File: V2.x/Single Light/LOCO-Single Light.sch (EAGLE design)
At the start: 32 parts, among them IC1 Atmega 328-P, IC2 MCP2515, IC3 MIC5219BM5, Q1 8MHz, Q2 16MHz

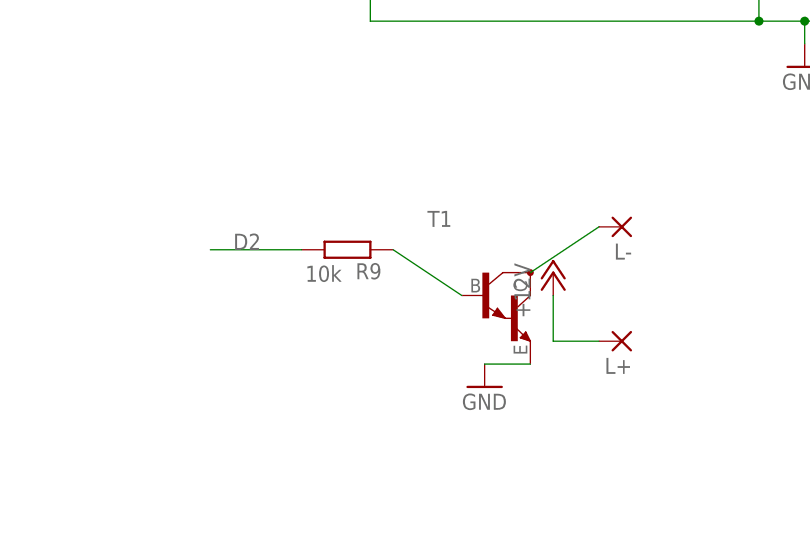
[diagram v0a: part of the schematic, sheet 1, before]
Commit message: initial
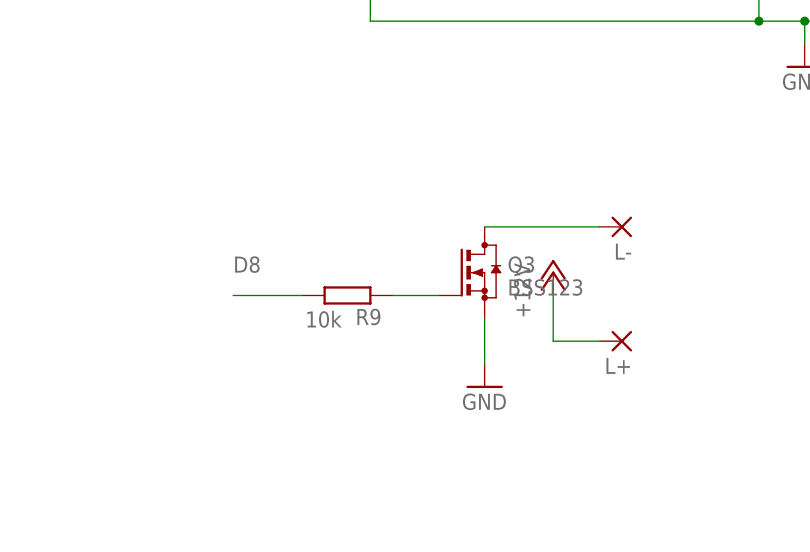
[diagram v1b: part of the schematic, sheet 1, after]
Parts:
- removed T1: (no value), transistor-neu-to92:MMBTA13LT1-NPN_DARL-SOT23-BEC
- added Q3: BSS123, transistor-small-signal:BSS123
- Q1, Q2: device crystal:CRYSTALHC49S -> crystal-geyer_V1_0:KX-9B
- R1, R15, R2, R9: device rcl:R-EU_R0603 -> rcl:R-EU_R0402
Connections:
- net D2: no longer R9.2
- net D8: now also R9.2
- net GND: now also Q3.S; no longer T1.E
- net LIGHT: now also Q3.D; no longer T1.C
- net N$2: now also Q3.G; no longer T1.B
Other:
- moved on the sheet: R9
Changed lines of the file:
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@@
 <part name="GND2" library="supply1" library_urn="urn:adsk.eagle:library:371" deviceset="GND" device=""/>
 <part name="P+2" library="supply1" library_urn="urn:adsk.eagle:library:371" deviceset="VCC" device=""/>
-<part name="R1" library="rcl" library_urn="urn:adsk.eagle:library:334" deviceset="R-EU_" device="R0603" package3d_urn="urn:adsk.eagle:package:23555/3" value="10k"/>
+<part name="R1" library="rcl" library_urn="urn:adsk.eagle:library:334" deviceset="R-EU_" device="R0402" package3d_urn="urn:adsk.eagle:package:23547/3" value="10k"/>
 <part name="C1" library="rcl" library_urn="urn:adsk.eagle:library:334" deviceset="C-EU" device="C0402K" package3d_urn="urn:adsk.eagle:package:23679/2" value="22p"/>
 <part name="C2" library="rcl" library_urn="urn:adsk.eagle:library:334" deviceset="C-EU" device="C0402K" package3d_urn="urn:adsk.eagle:package:23679/2" value="22p"/>
 <part name="GND3" library="supply1" library_urn="urn:adsk.eagle:library:371" deviceset="GND" device=""/>
-<part name="Q1" library="crystal" library_urn="urn:adsk.eagle:library:204" deviceset="CRYSTAL" device="HC49S" package3d_urn="urn:adsk.eagle:package:12071/1" value="8MHz"/>
+<part name="Q1" library="crystal-geyer_V1_0" library_urn="urn:adsk.eagle:library:203" deviceset="KX" device="-9B" package3d_urn="urn:adsk.eagle:package:11930/1" value="8MHz"/>
 <part name="C3" library="rcl" library_urn="urn:adsk.eagle:library:334" deviceset="C-EU" device="C0402K" package3d_urn="urn:adsk.eagle:package:23679/2" value="22p"/>
 <part name="C4" library="rcl" library_urn="urn:adsk.eagle:library:334" deviceset="C-EU" device="C0402K" package3d_urn="urn:adsk.eagle:package:23679/2" value="22p"/>
 <part name="GND4" library="supply1" library_urn="urn:adsk.eagle:library:371" deviceset="GND" device=""/>
-<part name="Q2" library="crystal" library_urn="urn:adsk.eagle:library:204" deviceset="CRYSTAL" device="HC49S" package3d_urn="urn:adsk.eagle:package:12071/1" value="16MHz"/>
-<part name="R2" library="rcl" library_urn="urn:adsk.eagle:library:334" deviceset="R-EU_" device="R0603" package3d_urn="urn:adsk.eagle:package:23555/3" value="10k"/>
+<part name="Q2" library="crystal-geyer_V1_0" library_urn="urn:adsk.eagle:library:203" deviceset="KX" device="-9B" package3d_urn="urn:adsk.eagle:package:11930/1" value="16MHz"/>
+<part name="R2" library="rcl" library_urn="urn:adsk.eagle:library:334" deviceset="R-EU_" device="R0402" package3d_urn="urn:adsk.eagle:package:23547/3" value="10k"/>
 <part name="C5" library="rcl" library_urn="urn:adsk.eagle:library:334" deviceset="C-EU" device="C0402K" package3d_urn="urn:adsk.eagle:package:23679/2" value="100n"/>
 <part name="IC1" library="atmel" library_urn="urn:adsk.eagle:library:105" deviceset="MEGA8" device="-AI" package3d_urn="urn:adsk.eagle:package:4313/2" value="Atmega 328-P"/>
@@
 <part name="C16" library="rcl" library_urn="urn:adsk.eagle:library:334" deviceset="CPOL-EU" device="A/3216-18W" package3d_urn="urn:adsk.eagle:package:23408/2" value="16uF"/>
 <part name="GND8" library="supply1" library_urn="urn:adsk.eagle:library:371" deviceset="GND" device=""/>
-<part name="R9" library="rcl" library_urn="urn:adsk.eagle:library:334" deviceset="R-EU_" device="R0603" package3d_urn="urn:adsk.eagle:package:23555/3" value="10k"/>
-<part name="R15" library="rcl" library_urn="urn:adsk.eagle:library:334" deviceset="R-EU_" device="R0603" package3d_urn="urn:adsk.eagle:package:23555/3" value="10k"/>
+<part name="R9" library="rcl" library_urn="urn:adsk.eagle:library:334" deviceset="R-EU_" device="R0402" package3d_urn="urn:adsk.eagle:package:23547/3" value="10k"/>
+<part name="R15" library="rcl" library_urn="urn:adsk.eagle:library:334" deviceset="R-EU_" device="R0402" package3d_urn="urn:adsk.eagle:package:23547/3" value="10k"/>
 <part name="+5V" library="led" library_urn="urn:adsk.eagle:library:259" deviceset="LED" device="CHIP-LED0603" package3d_urn="urn:adsk.eagle:package:15819/3"/>
 <part name="P+4" library="supply1" library_urn="urn:adsk.eagle:library:371" deviceset="+12V" device=""/>
@@
 <part name="L-" library="wirepad" library_urn="urn:adsk.eagle:library:412" deviceset="1,6/0,8" device="" package3d_urn="urn:adsk.eagle:package:30830/1"/>
 <part name="L+" library="wirepad" library_urn="urn:adsk.eagle:library:412" deviceset="1,6/0,8" device="" package3d_urn="urn:adsk.eagle:package:30830/1"/>
-<part name="T1" library="transistor-neu-to92" library_urn="urn:adsk.eagle:library:397" deviceset="*-NPN_DARL-" device="SOT23-BEC" package3d_urn="urn:adsk.eagle:package:28748/2" technology="MMBTA13LT1"/>
 <part name="GND5" library="supply1" library_urn="urn:adsk.eagle:library:371" deviceset="GND" device=""/>
 <part name="C-G" library="wirepad" library_urn="urn:adsk.eagle:library:412" deviceset="1,6/0,8" device="" package3d_urn="urn:adsk.eagle:package:30830/1"/>
@@
 <part name="IC3" library="v-reg-micrel" library_urn="urn:adsk.eagle:library:408" deviceset="MIC5219BM5" device="" package3d_urn="urn:adsk.eagle:package:30272/1"/>
 <part name="C7" library="rcl" library_urn="urn:adsk.eagle:library:334" deviceset="C-EU" device="C0402K" package3d_urn="urn:adsk.eagle:package:23679/2" value="470pF"/>
+<part name="Q3" library="transistor-small-signal" library_urn="urn:adsk.eagle:library:401" deviceset="BSS123" device="" package3d_urn="urn:adsk.eagle:package:28738/2"/>
 </parts>
 <sheets>
@@
 <attribute name="VALUE" x="53.34" y="-60.96" size="1.778" layer="96"/>
 </instance>
-<instance part="R9" gate="G$1" x="101.6" y="-30.48" smashed="yes" rot="R180" grouprefs="FET">
-<attribute name="NAME" x="105.41" y="-31.9786" size="1.778" layer="95" rot="R180"/>
-<attribute name="VALUE" x="100.965" y="-32.258" size="1.778" layer="96" rot="R180"/>
+<instance part="R9" gate="G$1" x="101.6" y="-35.56" smashed="yes" rot="R180" grouprefs="FET">
+<attribute name="NAME" x="105.41" y="-37.0586" size="1.778" layer="95" rot="R180"/>
+<attribute name="VALUE" x="100.965" y="-37.338" size="1.778" layer="96" rot="R180"/>
 </instance>
 <instance part="R15" gate="G$1" x="55.88" y="-45.72" smashed="yes" rot="R90" grouprefs="POWER">
@@
 <attribute name="VALUE" x="133.223" y="-37.338" size="1.778" layer="96" rot="R180"/>
 </instance>
-<instance part="T1" gate="G$1" x="116.84" y="-35.56" smashed="yes">
-<attribute name="NAME" x="110.49" y="-27.94" size="1.778" layer="95"/>
-<attribute name="VALUE" x="112.776" y="-30.48" size="1.778" layer="96"/>
-</instance>
 <instance part="GND5" gate="1" x="116.84" y="-45.72" smashed="yes" grouprefs="FET">
 <attribute name="VALUE" x="114.3" y="-48.26" size="1.778" layer="96"/>
@@
 <attribute name="NAME" x="-4.064" y="-46.101" size="1.778" layer="95" rot="R180"/>
 <attribute name="VALUE" x="-4.064" y="-41.021" size="1.778" layer="96" rot="R180"/>
+</instance>
+<instance part="Q3" gate="G$1" x="116.84" y="-33.02" smashed="yes">
+<attribute name="NAME" x="119.38" y="-33.02" size="1.778" layer="95"/>
+<attribute name="VALUE" x="119.38" y="-35.56" size="1.778" layer="96"/>
 </instance>
 </instances>
@@
 </segment>
 <segment>
-<wire x1="121.92" y1="-43.18" x2="116.84" y2="-43.18" width="0.1524" layer="91" grouprefs="FET"/>
-<pinref part="T1" gate="G$1" pin="E"/>
+<wire x1="116.84" y1="-38.1" x2="116.84" y2="-43.18" width="0.1524" layer="91" grouprefs="FET"/>
 <pinref part="GND5" gate="1" pin="GND"/>
+<pinref part="Q3" gate="G$1" pin="S"/>
 </segment>
 </net>
@@
 <pinref part="IC1" gate="G$1" pin="PB0(ICP)"/>
 </segment>
+<segment>
+<pinref part="R9" gate="G$1" pin="2"/>
+<wire x1="96.52" y1="-35.56" x2="88.9" y2="-35.56" width="0.1524" layer="91" grouprefs="FET"/>
+<label x="88.9" y="-33.02" size="1.778" layer="95" grouprefs="FET"/>
+</segment>
 </net>
 <net name="TX" class="0">
@@
 <wire x1="58.42" y1="45.72" x2="73.66" y2="45.72" width="0.1524" layer="91" grouprefs="MCU"/>
 <label x="68.58" y="45.72" size="1.778" layer="95" grouprefs="MCU"/>
-</segment>
-<segment>
-<pinref part="R9" gate="G$1" pin="2"/>
-<wire x1="96.52" y1="-30.48" x2="86.36" y2="-30.48" width="0.1524" layer="91" grouprefs="FET"/>
-<label x="88.9" y="-30.48" size="1.778" layer="95" grouprefs="FET"/>
 </segment>
 </net>
@@
 <net name="N$2" class="0">
 <segment>
-<wire x1="114.3" y1="-35.56" x2="106.68" y2="-30.48" width="0.1524" layer="91" grouprefs="FET"/>
+<wire x1="111.76" y1="-35.56" x2="106.68" y2="-35.56" width="0.1524" layer="91" grouprefs="FET"/>
 <pinref part="R9" gate="G$1" pin="1"/>
-<pinref part="T1" gate="G$1" pin="B"/>
+<pinref part="Q3" gate="G$1" pin="G"/>
 </segment>
 </net>
@@
 <net name="LIGHT" class="0">
 <segment>
-<wire x1="121.92" y1="-33.02" x2="129.54" y2="-27.94" width="0.1524" layer="91" grouprefs="FET"/>
+<wire x1="116.84" y1="-27.94" x2="129.54" y2="-27.94" width="0.1524" layer="91" grouprefs="FET"/>
 <pinref part="L-" gate="P" pin="P"/>
-<pinref part="T1" gate="G$1" pin="C"/>
-</segment>
-</net>
+<pinref part="Q3" gate="G$1" pin="D"/>
+</segment>
+</net>

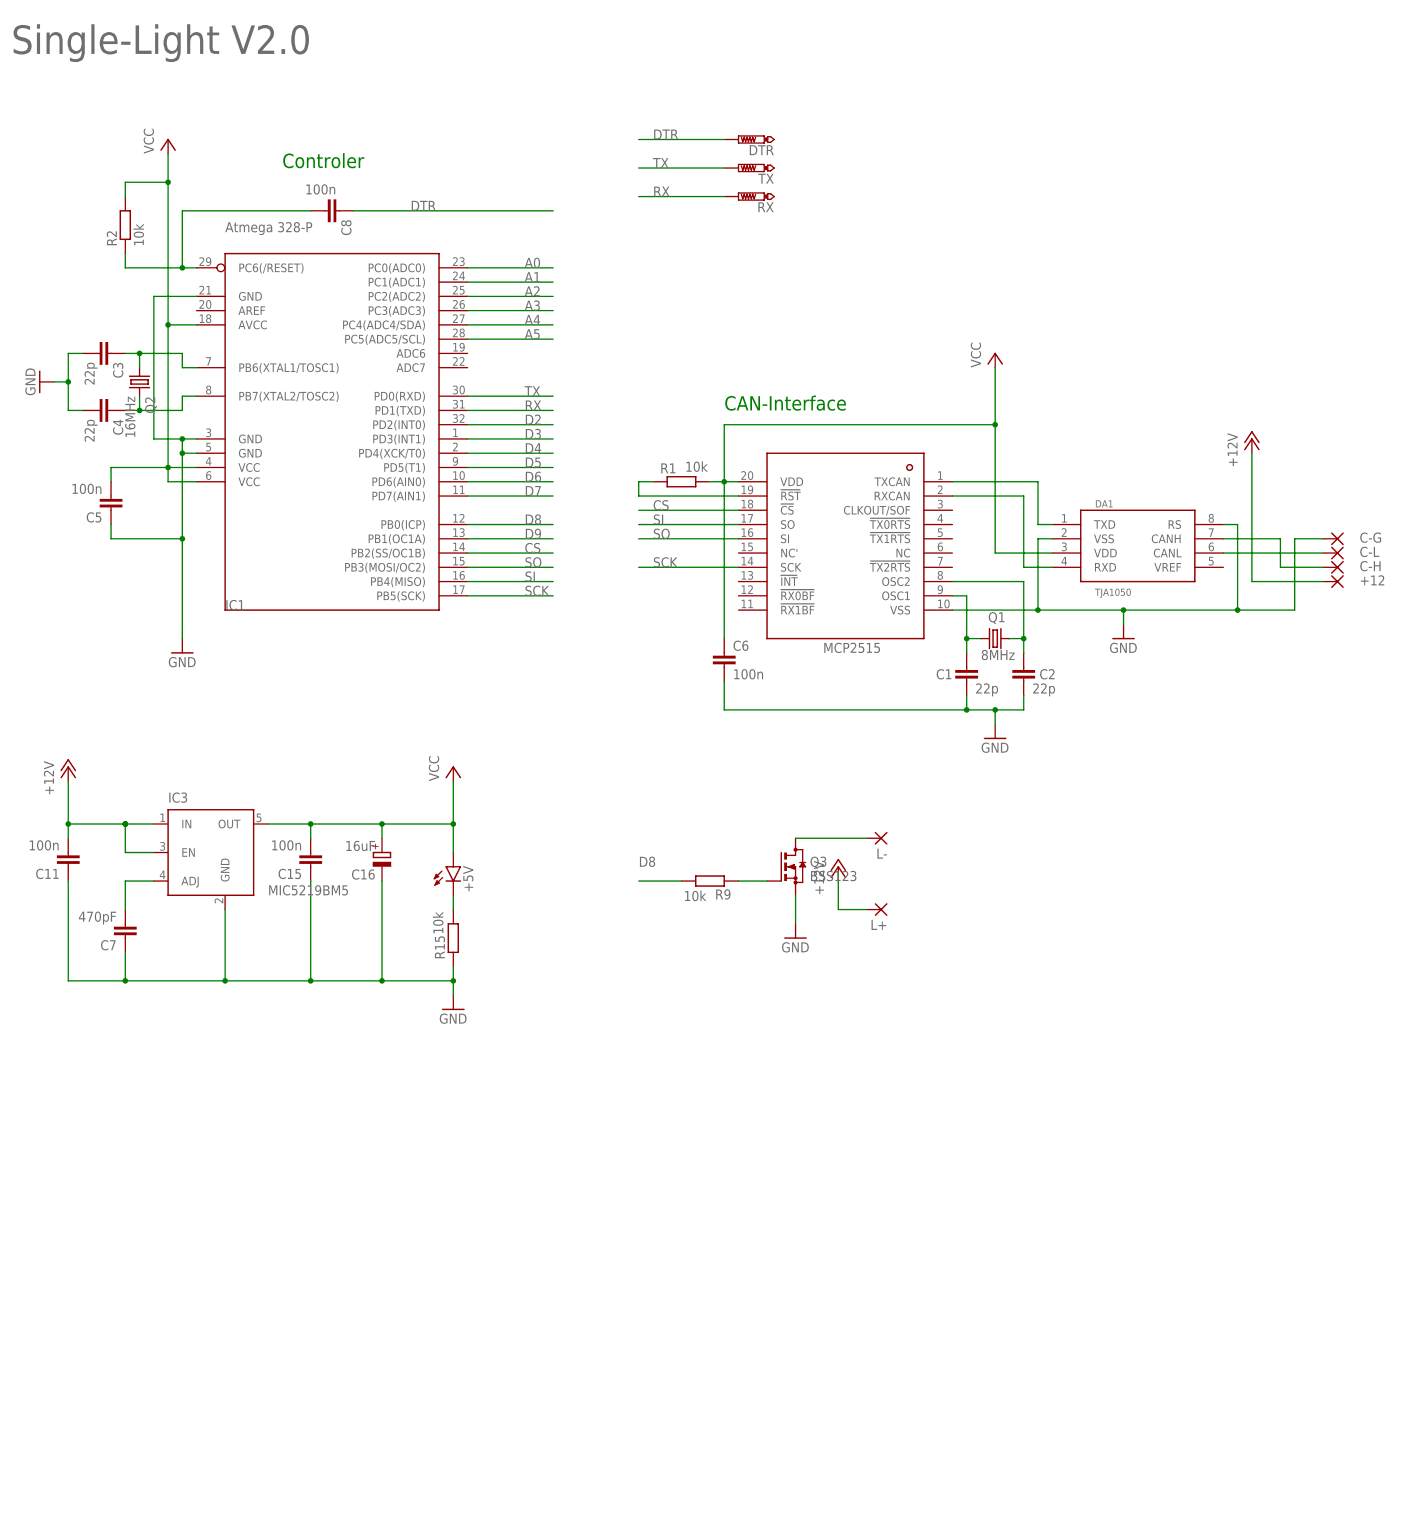
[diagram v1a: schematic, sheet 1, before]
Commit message: initial
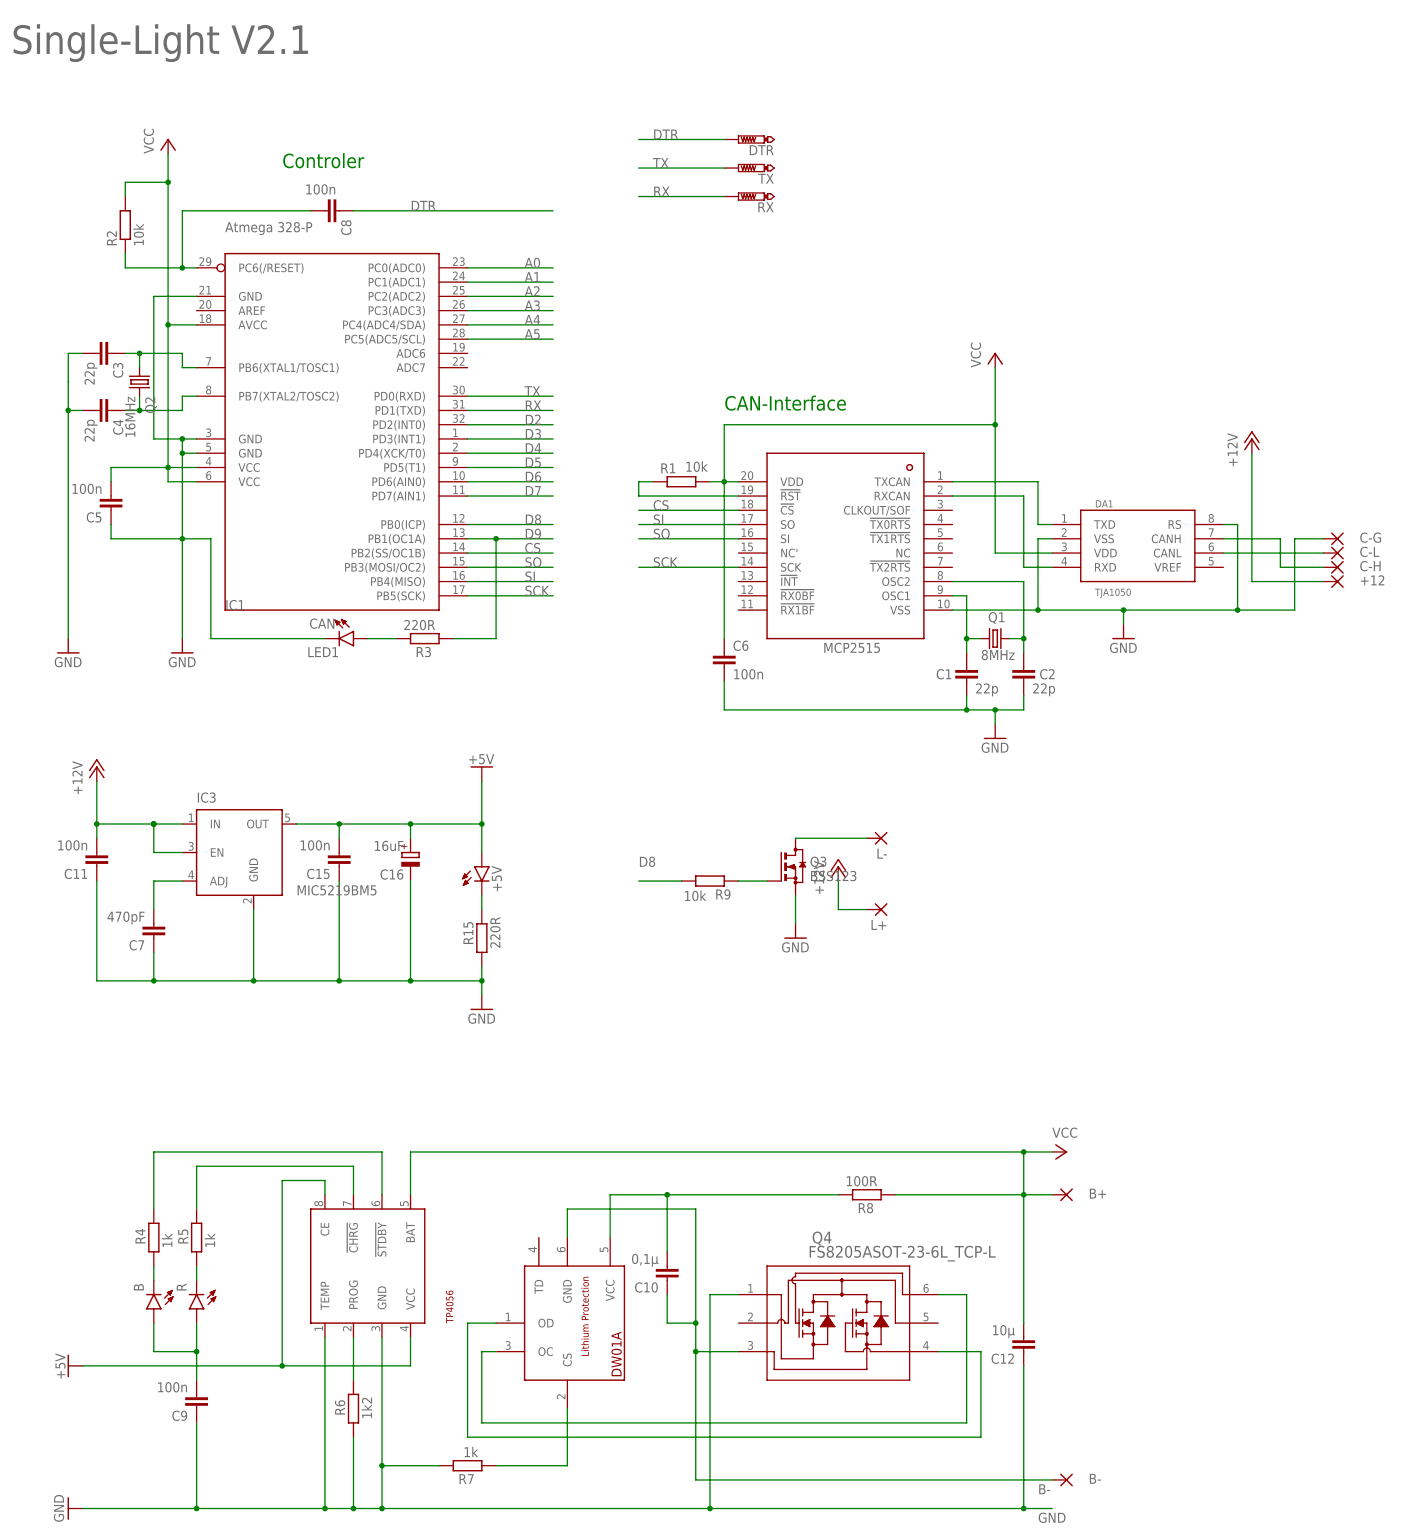
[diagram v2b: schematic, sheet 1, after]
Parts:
- added B, R: (no value), led:LEDCHIP-LED0603
- added B+, B-: (no value), wirepad:1,6/0,8
- added C10: 0,1µ, rcl:C-EUC0402K
- added C12: 10µ, rcl:C-EUC0402K
- added C9: 100n, rcl:C-EUC0402K
- added CAN: LED1, Opto-Electronic:LED_CHIP_BLUE-1608
- added IC4: TP4056, TP4056:TP4056
- added IC5: DW01A, DW01a:DW01A
- added Q4: FS8205ASOT-23-6L_TCP-L, FS8205A:FS8205ASOT-23-6L_TCP-L
- added R3: 220R, rcl:R-EU_R0402
- added R4, R5, R7: 1k, rcl:R-EU_R0402
- added R6: 1k2, rcl:R-EU_R0402
- added R8: 100R, rcl:R-EU_R0402
- R15: value 10k -> 220R
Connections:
- new net +5V: +5V.A, C15.2, C16.+, IC3.OUT, IC4.CE, IC4.VCC
- new net B-: B-.P, C10.1, IC5.GND, Q4.3
- new net N$13: B.A, C9.2, R.A
- new net N$14: IC5.OC, Q4.6
- new net N$16: IC5.OD, Q4.4
- new net N$17: C10.2, IC5.VCC, R8.2
- new net N$18: IC5.CS, R7.1
- new net N$3: CAN.A, R3.2
- new net N$4: B.C, R4.1
- new net N$5: R.C, R5.1
- new net N$7: IC4.!STDBY, R4.2
- new net N$8: IC4.!CHRG, R5.2
- new net N$9: IC4.PROG, R6.2
- net D9: now also R3.1
- net GND: now also C12.1, C9.1, CAN.C, IC4.GND, IC4.TEMP, Q4.1, R6.1, R7.2
- net VCC: now also B+.P, C12.2, IC4.BAT, R8.1; no longer +5V.A, C15.2, C16.+, IC3.OUT
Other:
- note added: "Single-Light V2.1"
- note removed: "Single-Light V2.0"
- moved on the sheet: +5V, C11, C15, C16, C7, IC3, R15
